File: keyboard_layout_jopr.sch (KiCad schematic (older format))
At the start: 229 parts, among them SW1 SW_Push, U1 ATmega32U4-AU, U2 SOT65P210X110, Y1 16MHz

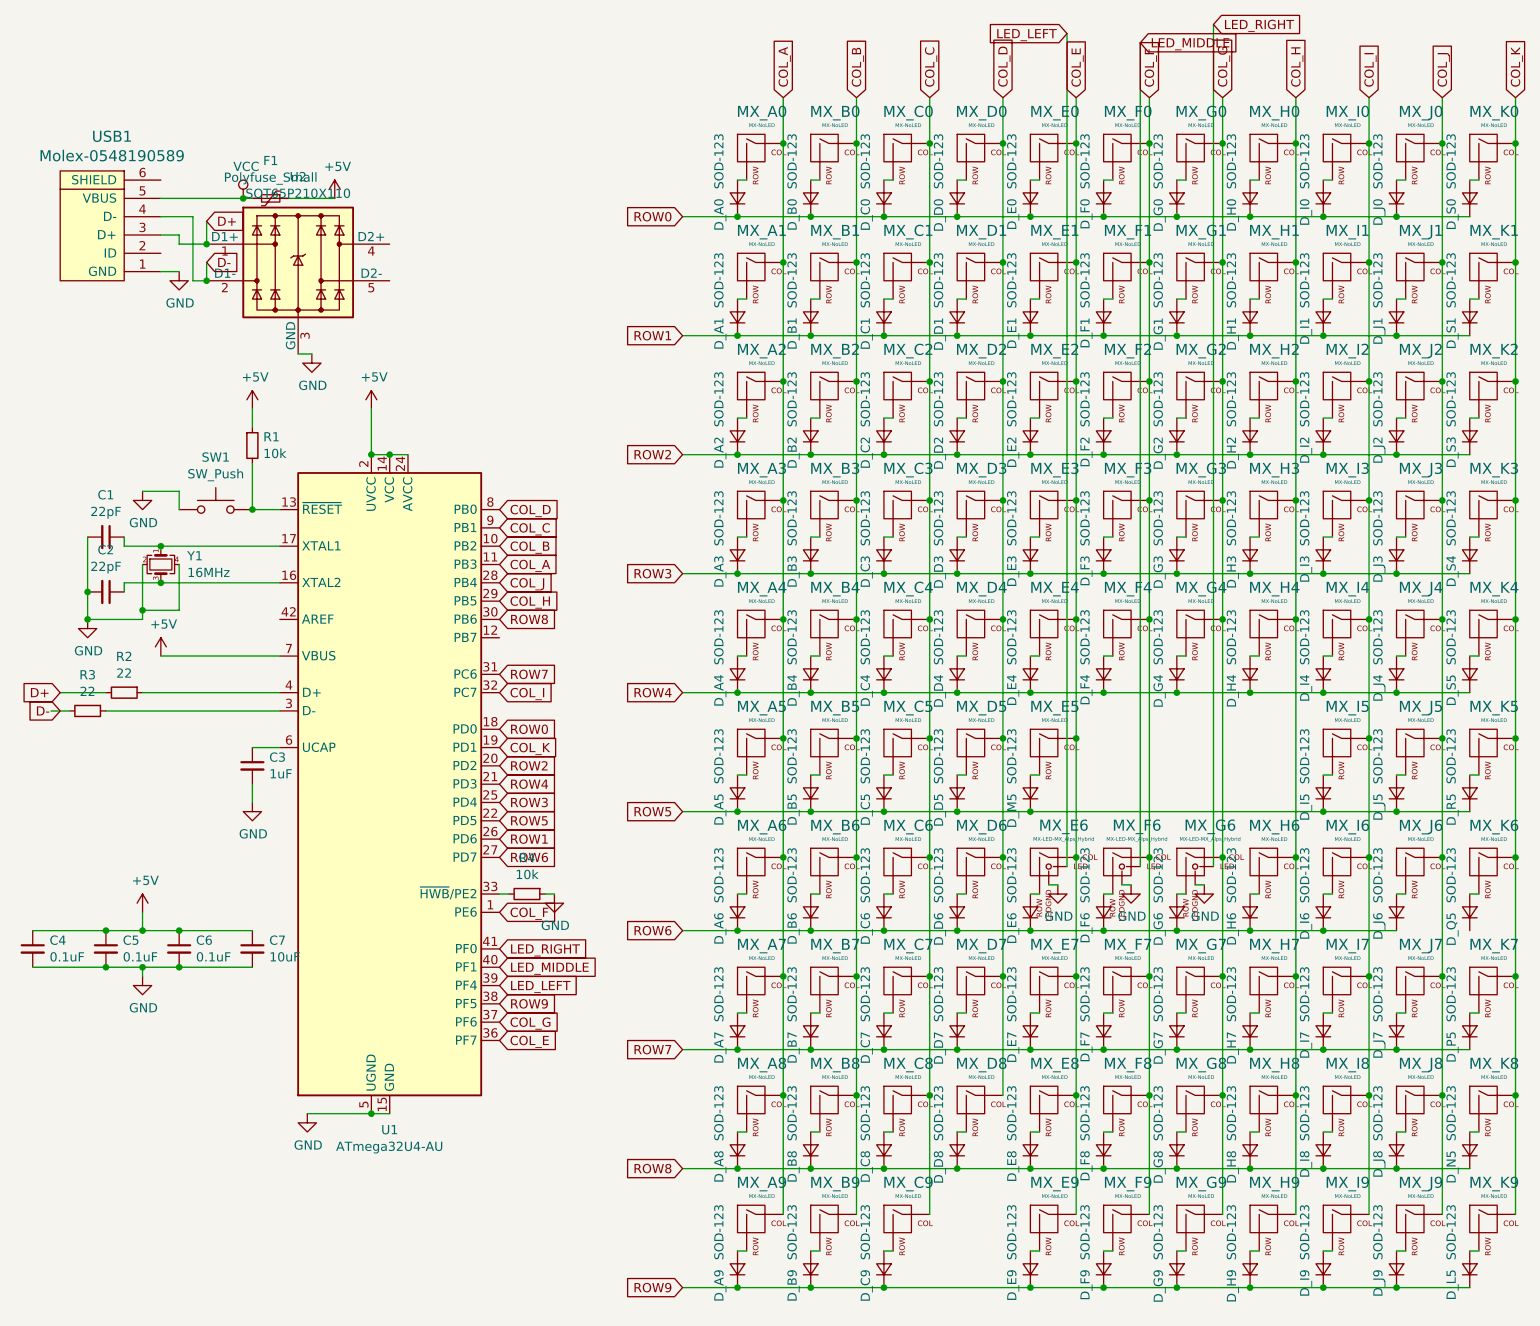
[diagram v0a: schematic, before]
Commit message: removed NumLock
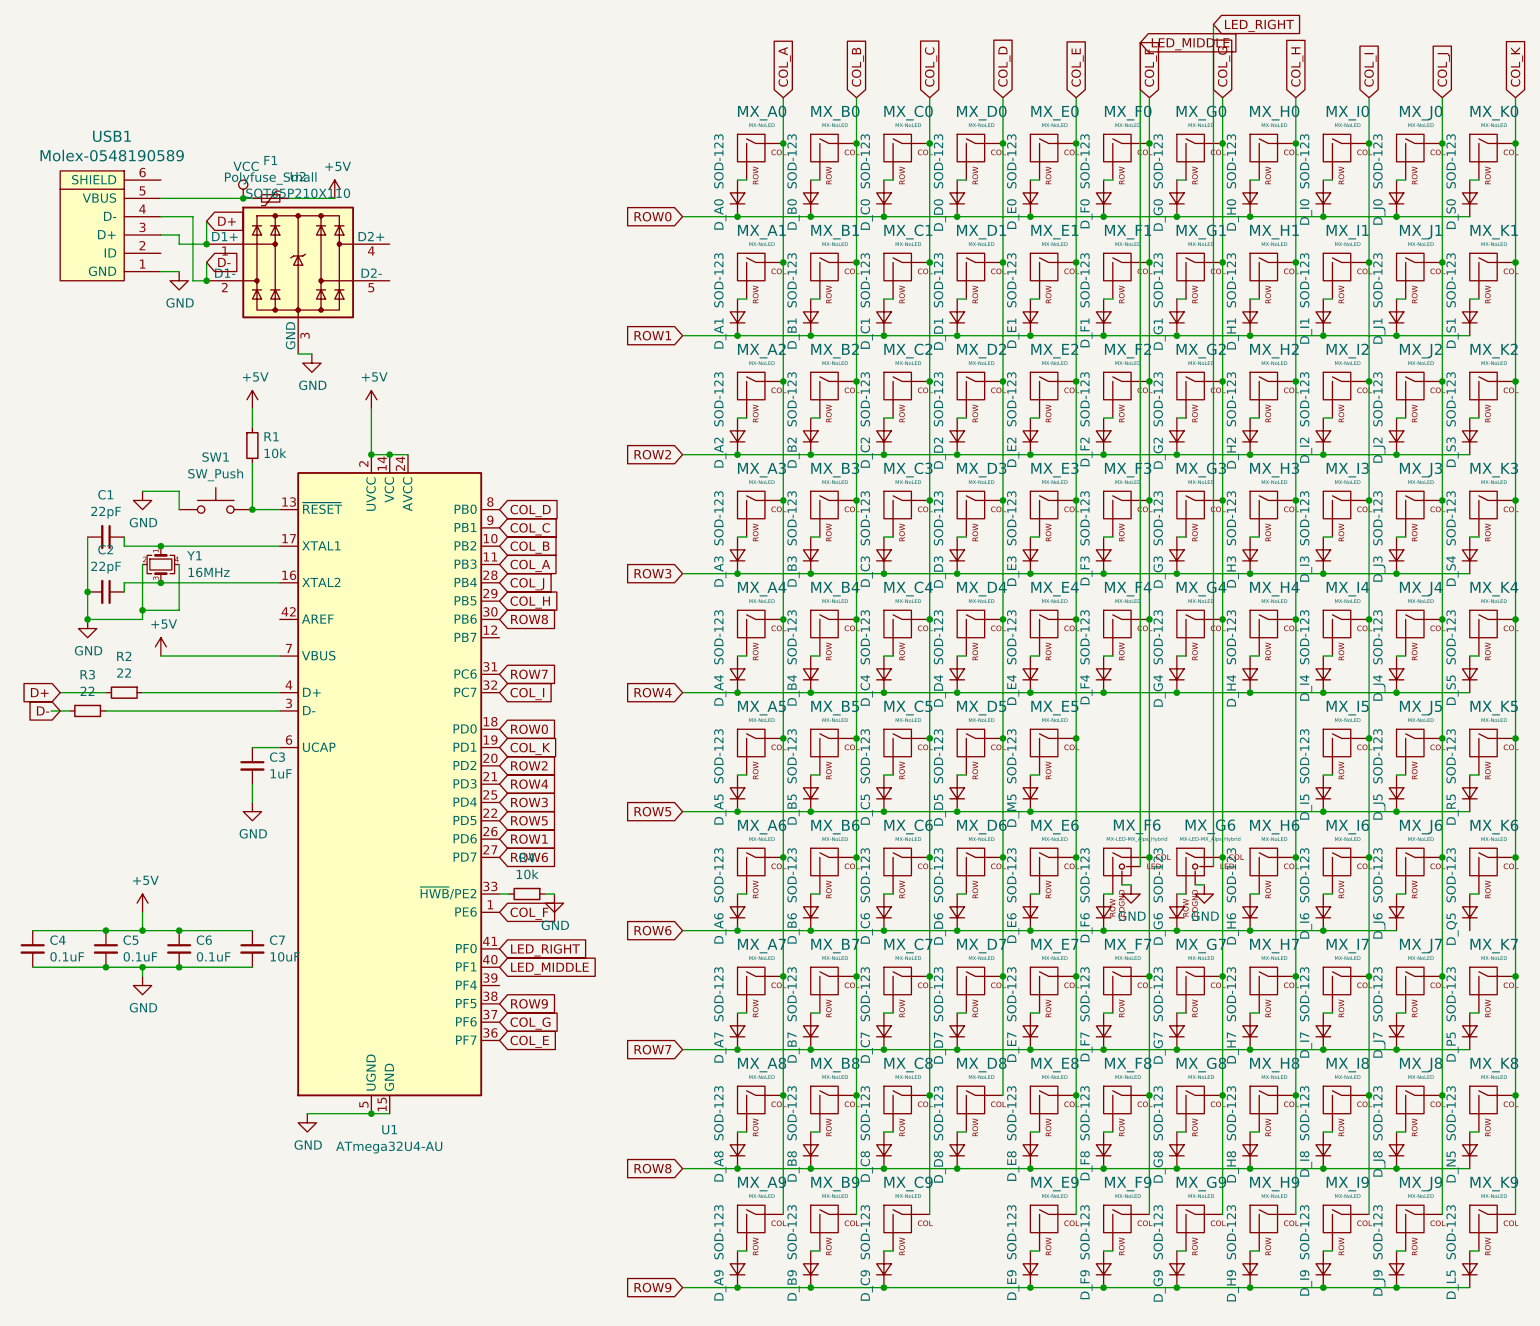
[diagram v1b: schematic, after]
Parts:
- removed MX_E6: MX-LED-MX_Alps_Hybrid, MX_Only:MXOnly-1U-FLIPPED, symbol keyboard_layout_jopr-rescue:MX-LED-MX_Alps_Hybrid
- added MX_E6: MX-NoLED, MX_Only:MXOnly-1U-NoLED, symbol keyboard_layout_jopr-rescue:MX-NoLED-MX_Alps_Hybrid
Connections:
- net COL_E: now also MX_E6.1 (COL)
- net at D_E6.2 (A): now also MX_E6.2 (ROW)
- net LED_LEFT: no longer names the net of U1.39 (PF4)
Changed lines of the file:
@@
 Connection ~ 1550 1450
-Wire Wire Line
-	6300 3950 6300 4600
 Wire Wire Line
 	6700 3300 6700 4600
 Wire Wire Line
 	7100 3300 7100 4600
-$Comp
-L keyboard_layout_jopr-rescue:MX-LED-MX_Alps_Hybrid MX_E6
-U 1 1 5D1102C1
-P 6150 4650
-F 0 "MX_E6" H 6232 4874 60  0000 C CNN
-F 1 "MX-LED-MX_Alps_Hybrid" H 6232 4800 20  0000 C CNN
-F 2 "MX_Only:MXOnly-1U-FLIPPED" H 5525 4625 60  0001 C CNN
-F 3 "" H 5525 4625 60  0001 C CNN
-	1    6150 4650
-	1    0    0    -1
-$EndComp
-Connection ~ 6300 4600
-Wire Wire Line
-	6300 4600 6300 5250
 $Comp
 L keyboard_layout_jopr-rescue:MX-LED-MX_Alps_Hybrid MX_F6
@@
 	1    0    0    -1
 $EndComp
-$Comp
-L power:GND #PWR0104
-U 1 1 5D11AF82
-P 6200 4750
-F 0 "#PWR0104" H 6200 4500 50  0001 C CNN
-F 1 "GND" H 6205 4577 50  0000 C CNN
-F 2 "" H 6200 4750 50  0001 C CNN
-F 3 "" H 6200 4750 50  0001 C CNN
-	1    6200 4750
-	1    0    0    -1
-$EndComp
-Wire Wire Line
-	6150 4750 6200 4750
 Wire Wire Line
 	6550 4750 6600 4750
 Wire Wire Line
 	6950 4750 7000 4750
-Wire Wire Line
-	6250 4650 6250 100
-Text GLabel 6250 100  0    50   Input ~ 0
-LED_LEFT
 Wire Wire Line
 	6650 4650 6650 150
@@
 Text GLabel 7050 50   2    50   Input ~ 0
 LED_RIGHT
-Text GLabel 3150 5300 2    50   Input ~ 0
-LED_LEFT
 Text GLabel 3150 5200 2    50   Input ~ 0
 LED_MIDDLE
 Text GLabel 3150 5100 2    50   Input ~ 0
 LED_RIGHT
+Wire Wire Line
+	6300 3950 6300 4600
+$Comp
+L keyboard_layout_jopr-rescue:MX-NoLED-MX_Alps_Hybrid MX_E6
+U 1 1 5D2D876E
+P 6150 4650
+F 0 "MX_E6" H 6183 4873 60  0000 C CNN
+F 1 "MX-NoLED" H 6183 4799 20  0000 C CNN
+F 2 "MX_Only:MXOnly-1U-NoLED" H 5525 4625 60  0001 C CNN
+F 3 "" H 5525 4625 60  0001 C CNN
+	1    6150 4650
+	1    0    0    -1
+$EndComp
+Connection ~ 6300 4600
+Wire Wire Line
+	6300 4600 6300 5250
 $EndSCHEMATC
